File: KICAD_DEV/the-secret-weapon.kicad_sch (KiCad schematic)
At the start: 5 parts, among them U1 STM32H757IITx

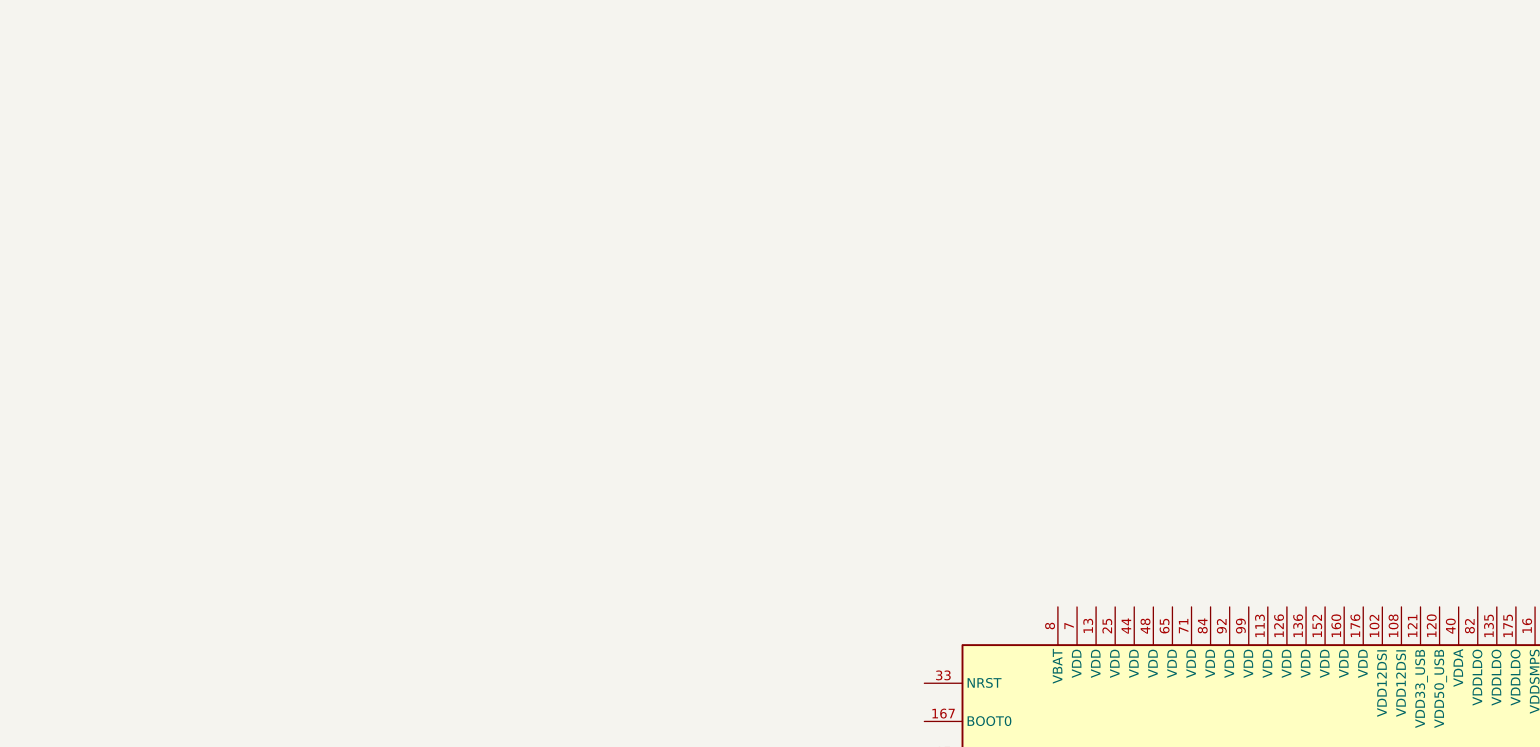
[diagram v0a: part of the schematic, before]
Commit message: working on USB PD
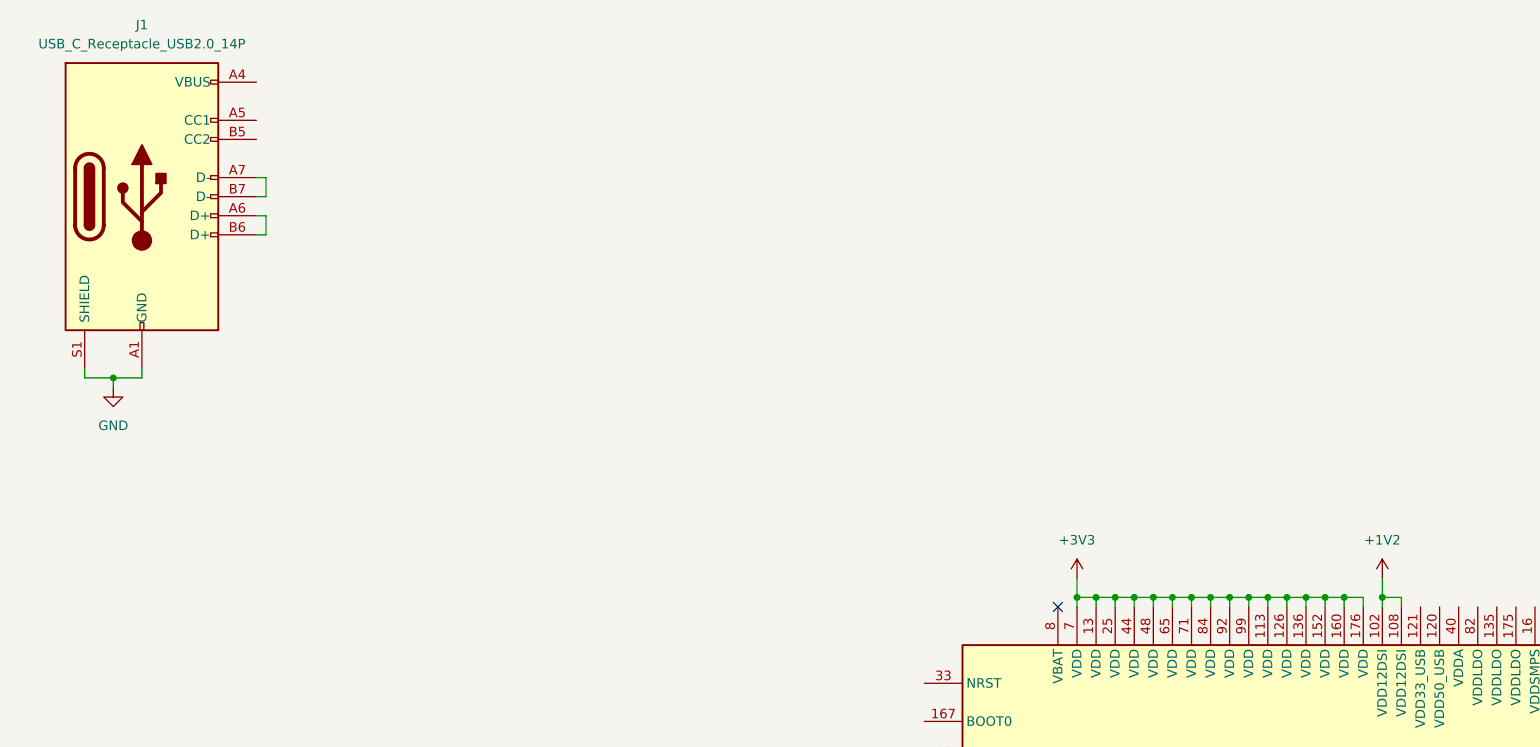
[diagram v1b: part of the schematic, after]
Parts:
- added J1: USB_C_Receptacle_USB2.0_14P, symbol Connector:USB_C_Receptacle_USB2.0_14P
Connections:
- net GND: now also J1.A1 (GND), J1.A12 (GND), J1.B1 (GND), J1.B12 (GND), J1.S1 (SHIELD)
- net +1V2: now reaches U1.102 (VDD12DSI)
- net +1V2: now also U1.108 (VDD12DSI)
- net +3V3: now reaches U1.113 (VDD)
- net +3V3: now also U1.126 (VDD), U1.13 (VDD), U1.136 (VDD), U1.152 (VDD), U1.160 (VDD), U1.176 (VDD), U1.25 (VDD), U1.44 (VDD), U1.48 (VDD), U1.65 (VDD), U1.7 (VDD), U1.71 (VDD), U1.84 (VDD), U1.92 (VDD), U1.99 (VDD)
- new net: J1.A4 (VBUS), J1.A9 (VBUS), J1.B4 (VBUS), J1.B9 (VBUS)
- new net: J1.A6 (D+), J1.B6 (D+)
- new net: J1.A7 (D-), J1.B7 (D-)
- no-connect marks 0 -> 1
